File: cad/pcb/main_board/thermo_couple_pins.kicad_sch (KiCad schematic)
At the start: 3 parts

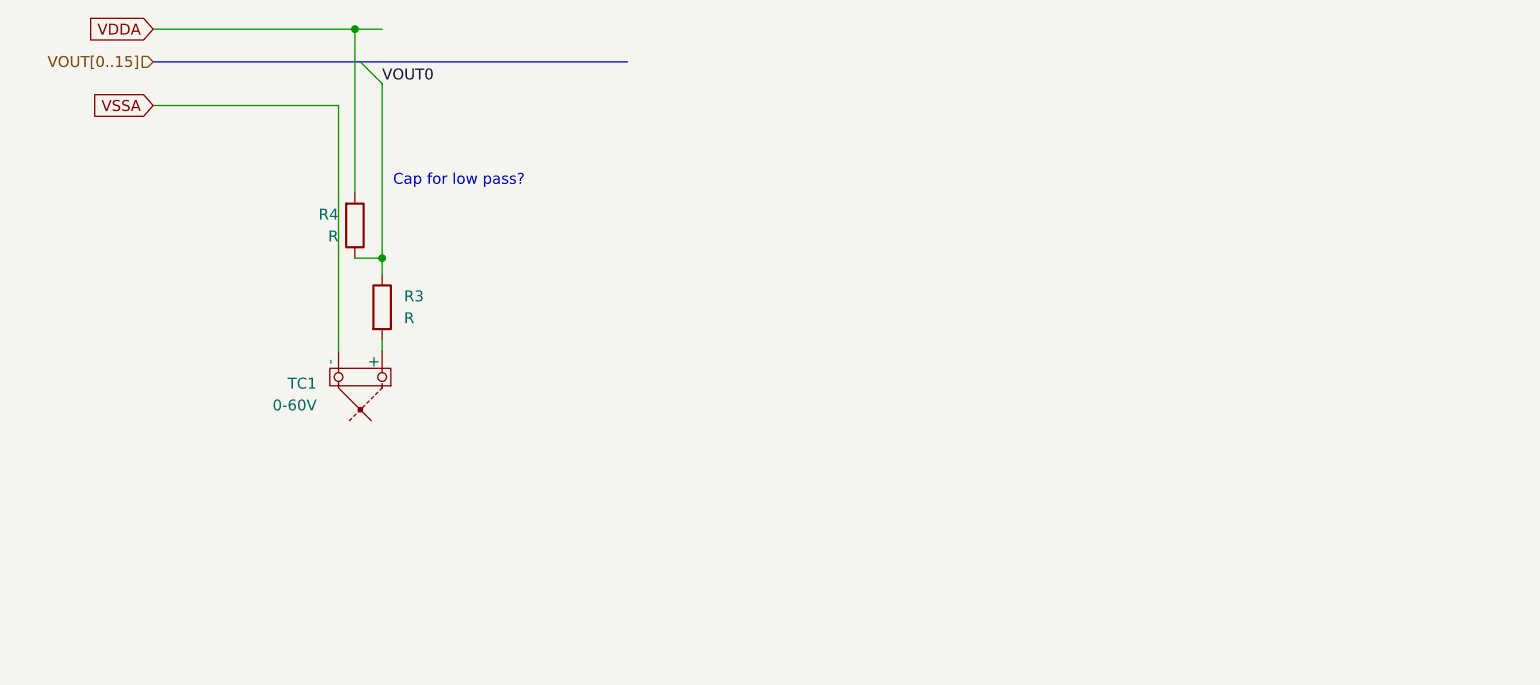
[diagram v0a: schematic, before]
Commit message: Thermo Couple Pins
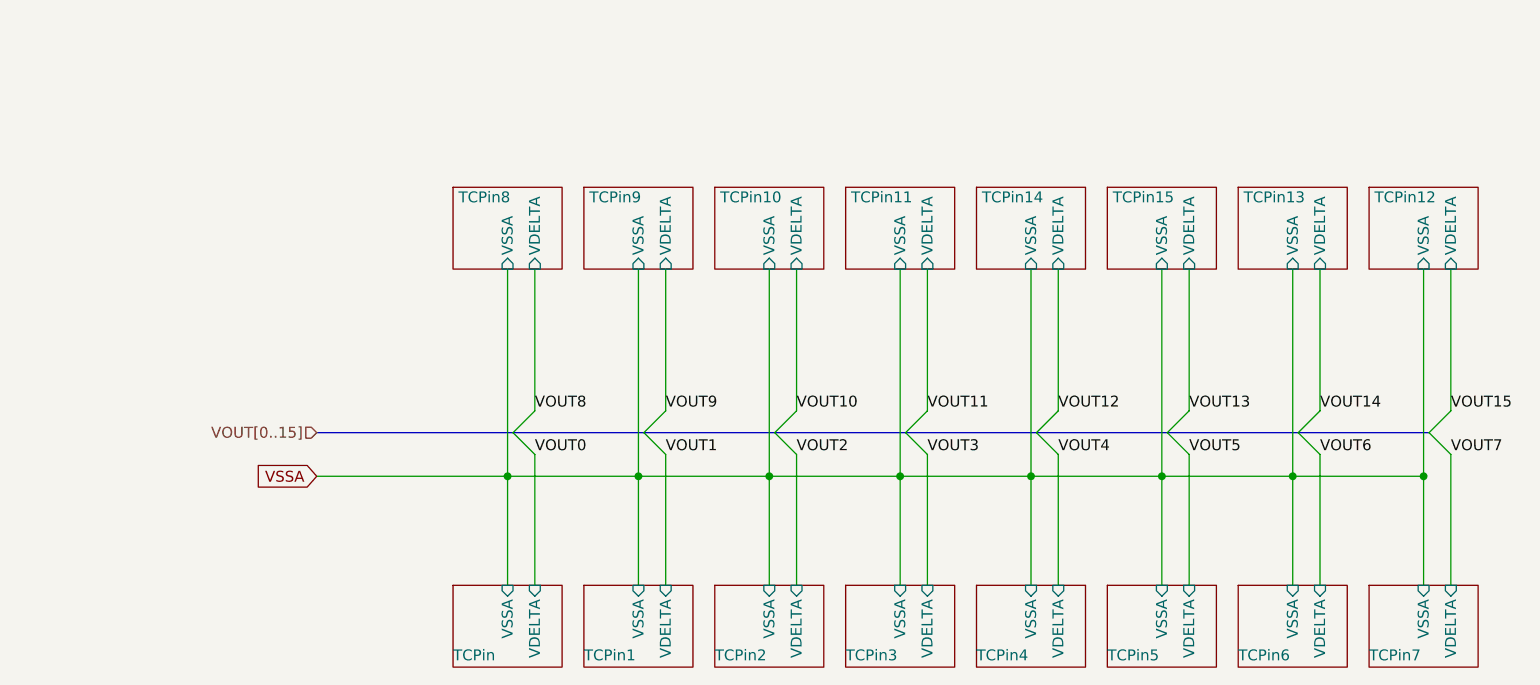
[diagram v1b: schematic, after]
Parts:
- removed R3, R4: R, symbol Device:R
- removed TC1: 0-60V, symbol Device:Thermocouple_Block
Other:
- added sheet TCPin (tcpin.kicad_sch)
- added sheet TCPin1 (tcpin.kicad_sch)
- added sheet TCPin10 (tcpin.kicad_sch)
- added sheet TCPin11 (tcpin.kicad_sch)
- added sheet TCPin12 (tcpin.kicad_sch)
- added sheet TCPin13 (tcpin.kicad_sch)
- added sheet TCPin14 (tcpin.kicad_sch)
- added sheet TCPin15 (tcpin.kicad_sch)
- added sheet TCPin2 (tcpin.kicad_sch)
- added sheet TCPin3 (tcpin.kicad_sch)
- added sheet TCPin4 (tcpin.kicad_sch)
- added sheet TCPin5 (tcpin.kicad_sch)
- added sheet TCPin6 (tcpin.kicad_sch)
- added sheet TCPin7 (tcpin.kicad_sch)
- added sheet TCPin8 (tcpin.kicad_sch)
- added sheet TCPin9 (tcpin.kicad_sch)
- note removed: "Cap for low pass?"
